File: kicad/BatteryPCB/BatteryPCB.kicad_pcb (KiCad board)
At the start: 2 copper layers, 109.5 x 53.5 mm, 36 parts, among them J1 USB4105-GF-A, J2 BoostV, J3 BatteryV, J4 24V, J5 5V, J6 B3B-XH-A, U5 TPS7A4901DGNT, U7 MT3608, U8 TP4056

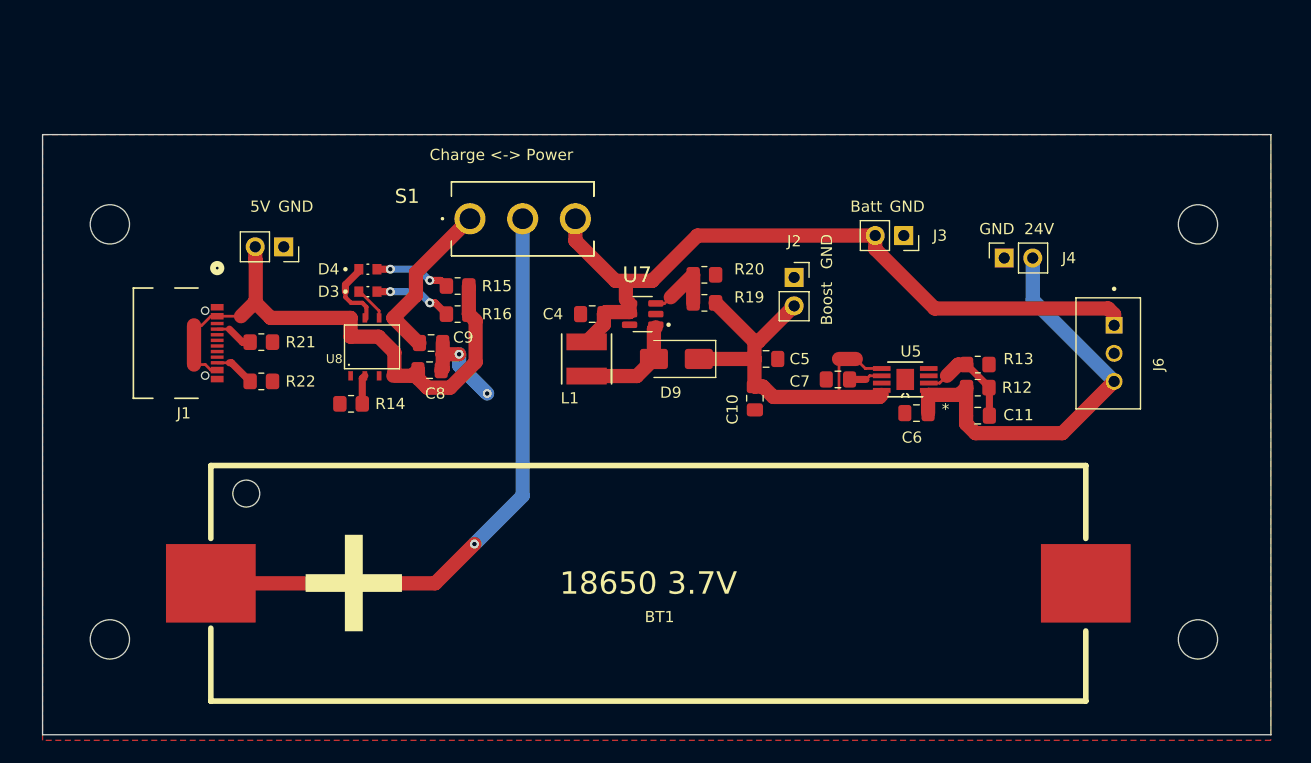
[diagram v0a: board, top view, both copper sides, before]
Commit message: Final PCB
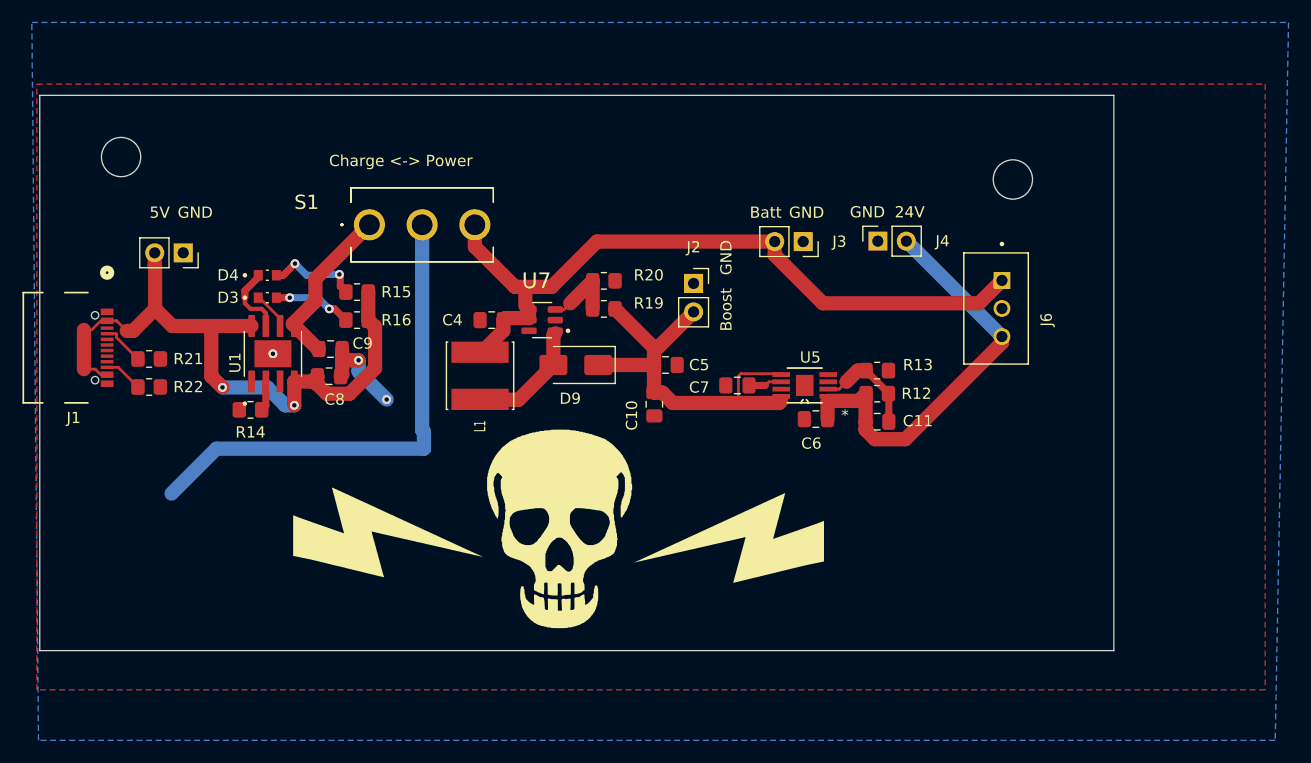
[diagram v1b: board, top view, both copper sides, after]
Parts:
- removed BT1: BK-18650-PC2, FreddyBattery:BH-18650-B1BA002
- removed H3, H4: MountingHole, MountingHole:MountingHole_3.5mm
- removed U8: TP4056, TP4056:SOT23-8
- added U1: TP4056, TP4056:SOP127P600X175-9N, F.Cu at (68.5, 115.5)
- L1: value 10µH -> VLS6045EX-100M; footprint SRN4018_4R7M:IND_BOURNS_SRN4018 -> VLS6045EX_100M:IND_VLS6045EX-100M
- R16: value 1k -> 470
- moved H1 17.0 mm to (134.5, 100.0)
- moved J4 11.4 mm to (122.5, 105.5)
- moved J6 10.8 mm to (133.0, 111.5)
- moved R21 10.1 mm to (57.5, 116.0)
- moved R22 10.0 mm to (57.5, 118.5)
- moved J1 9.82 mm to (50.3, 115.0)
- moved L1 9.62 mm to (87.0, 117.5), turned to -90 degrees
- moved C9 8.98 mm to (73.7, 115.1)
- moved C10 8.98 mm to (102.5, 120.0)
- moved C4 8.98 mm to (88.0, 112.5)
- moved C5 8.98 mm to (103.5, 116.5)
- moved C6 8.98 mm to (116.9, 121.4)
- moved C7 8.98 mm to (109.9, 118.4)
- moved C8 8.98 mm to (73.5, 117.5)
- moved D3 8.98 mm to (68.0, 110.5)
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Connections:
- D3 pad C: Net-(U8-~{STDBY}) -> /Battery&Charging/STDBY
- D4 pad C: Net-(U8-~{CHRG}) -> /Battery&Charging/CHRG
- L1 pad 1: Net-(D9-A) -> Battery_Voltage
- L1 pad 2: Battery_Voltage -> Net-(D9-A)
- U7 pad 6: (no net) -> unconnected-(U7-NC-Pad6)
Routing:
- net Net-(S1-COM): track 55.7 -> 44.2 mm, vias 1 -> 0
- net /Battery&Charging/VBUS_USB: track 50.9 -> 57.6 mm, vias 0 -> 2
- net /Battery&Charging/CHRG: track 0.00 -> 6.27 mm
- net Net-(U8-~{CHRG}): track 6.27 -> 0.00 mm
- net Net-(U8-~{STDBY}): track 3.15 -> 0.00 mm
- net /Battery&Charging/STDBY: track 0.00 -> 3.15 mm
- net Battery_Voltage: track 65.7 -> 63.9 mm
- net Net-(D4-PadA): track 6.81 -> 8.32 mm
- net /Battery&Charging/Boost_LDO_Point: track 38.2 -> 36.9 mm
- net Net-(D9-A): track 9.53 -> 10.7 mm
- net +24V: track 37.9 -> 37.1 mm
- net GND: vias 2 -> 3
- added copper zone on B.Cu, net GND
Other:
- board size 109.5 x 53.5 mm -> 95.8 x 49.5 mm
